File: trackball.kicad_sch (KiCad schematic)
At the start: 174 parts, among them J1 ZX-PM2.0-2-4PY, SW1 HX TC-5608-Y, SW2 HX TC-5608-Y, SW3 HX TC-5608-Y, SW4 HX TC-5608-Y, SW5 HX TC-5608-Y, SW6 HX TC-5608-Y, SW7 HX TC-5608-Y, SW8 HX TC-5608-Y, U1 SY8089A1AAC, U10 WS2812B, U11 WS2812B, U12 WS2812B, U13 WS2812B, U14 WS2812B, U15 WS2812B, U16 WS2812B, U17 WS2812B, U18 WS2812B, U19 WS2812B, U2 USB-TYPE-C-017, U20 WS2812B, U3 PMW3610, U4 PMW3610, U5 WS2812B, U6 WS2812B, U7 WS2812B, U8 WS2812B, U9 WS2812B, X1 XL7EL89CKI-111YLC-32M

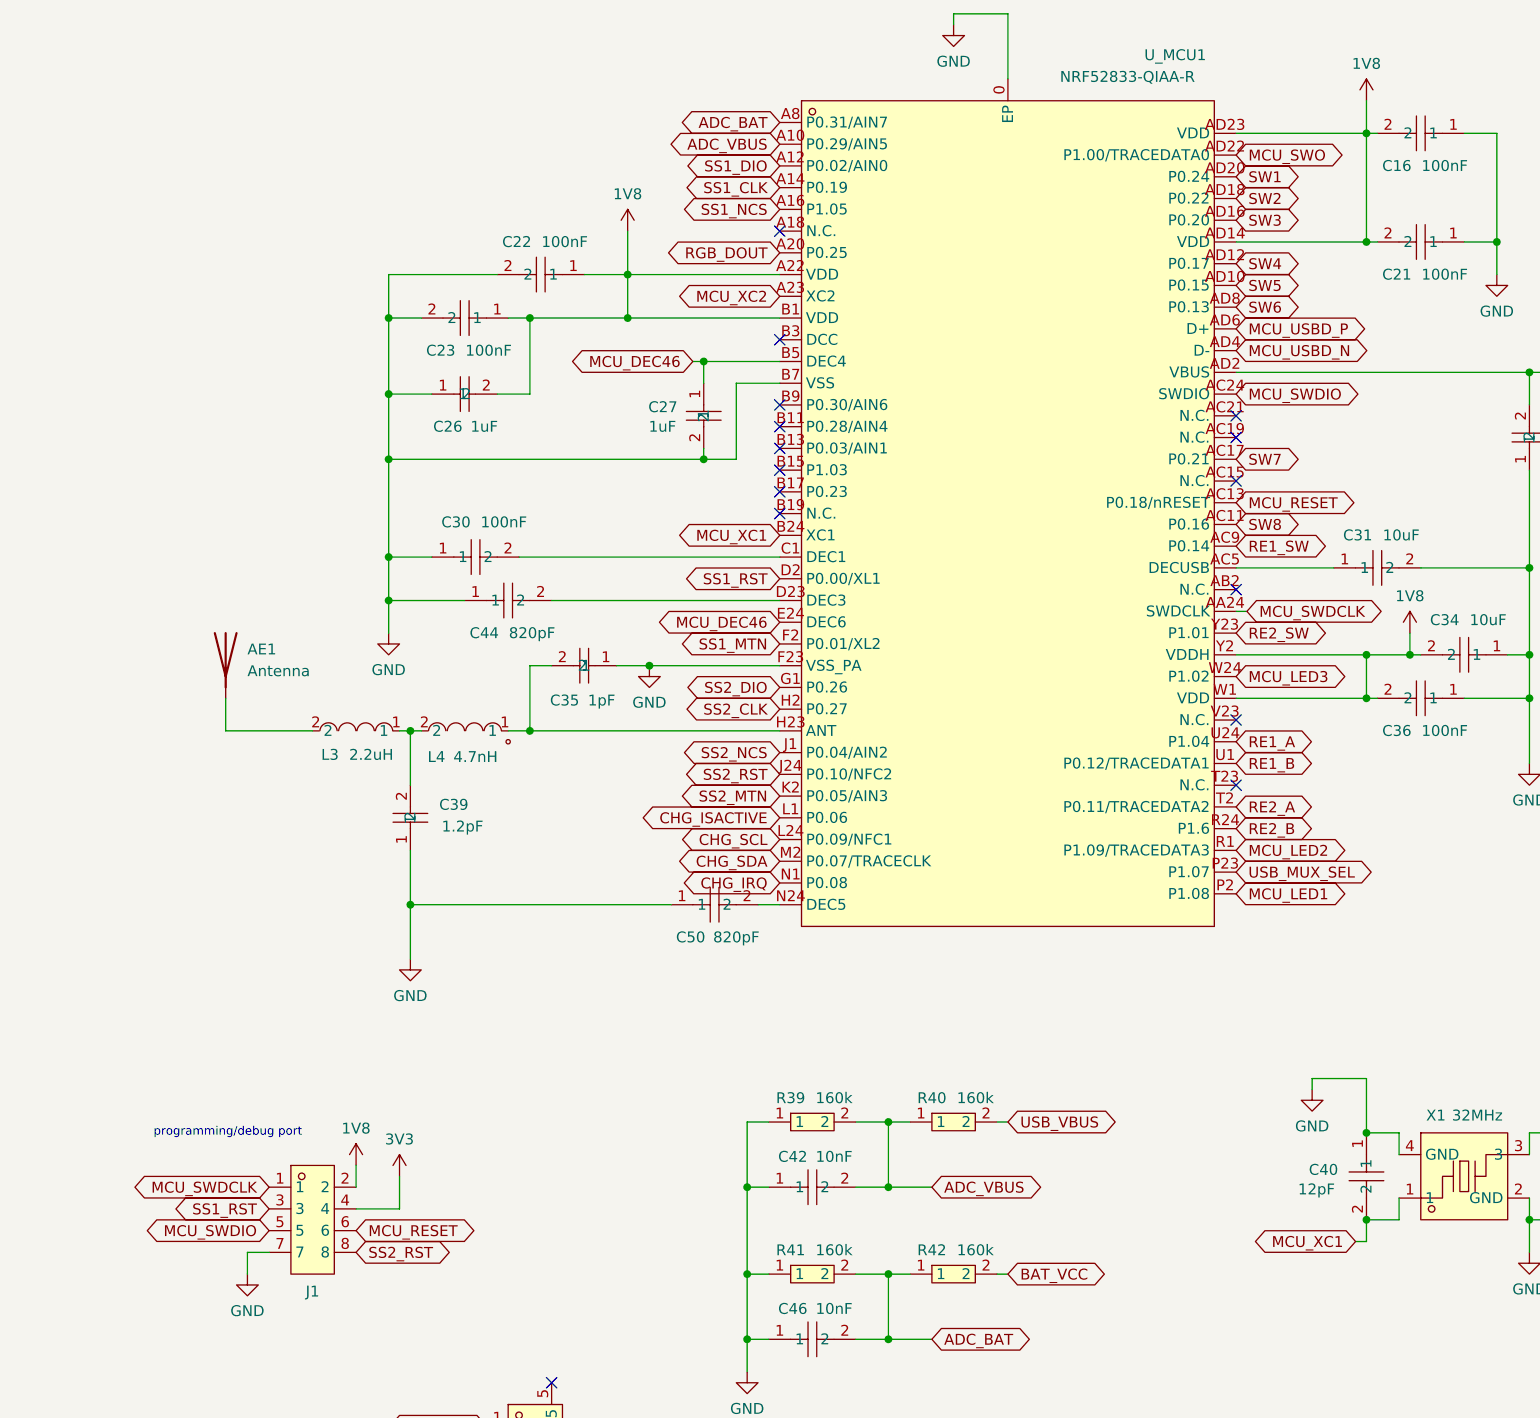
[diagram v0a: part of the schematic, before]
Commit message: chore: checkpoint
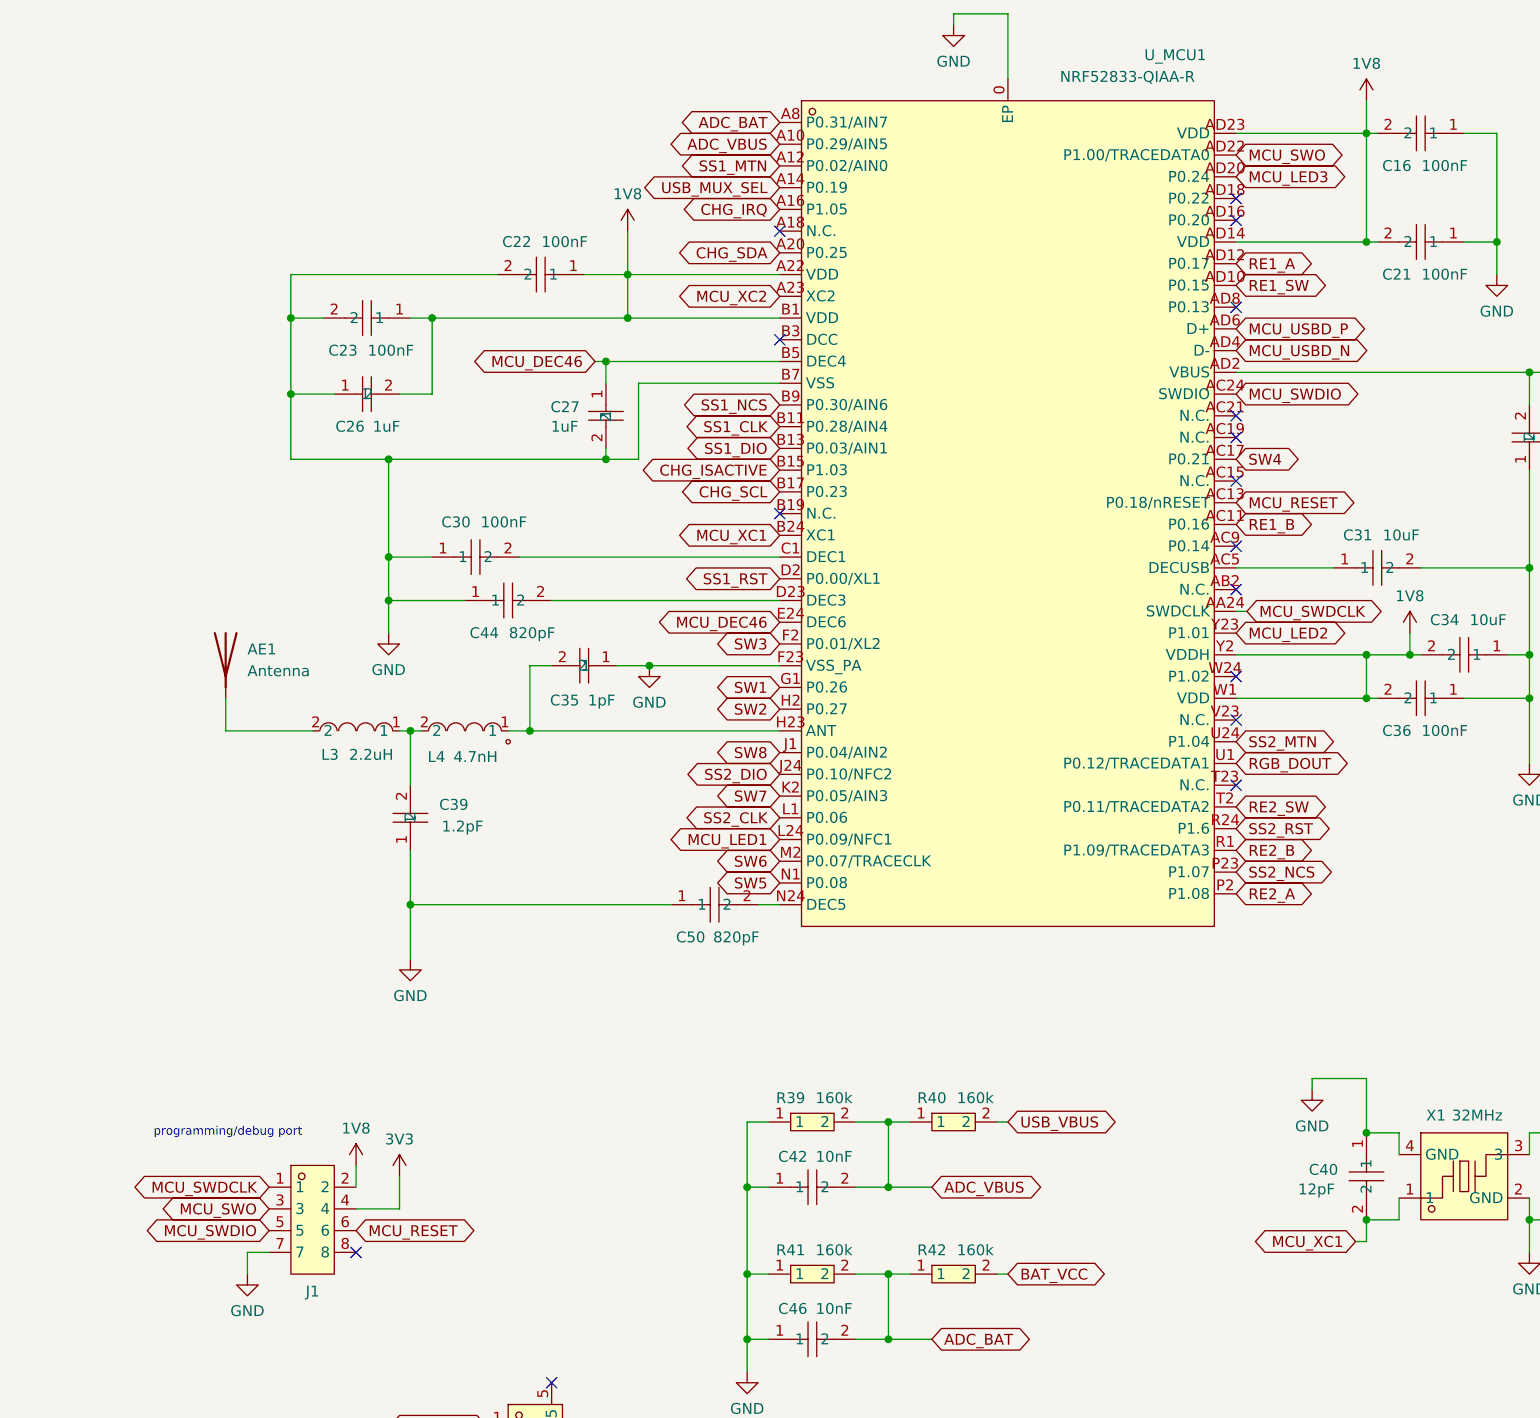
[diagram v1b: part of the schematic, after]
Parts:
- AE1: footprint antenna:Texas_SWRA117D_2.4GHz_Right -> antenna:Texas_SWRA117D_2.4GHz_Left
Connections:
- net CHG_IRQ: now also U_MCU1.A16 (P1.05); no longer U_MCU1.N1 (P0.08)
- net CHG_ISACTIVE: now also U_MCU1.B15 (P1.03); no longer U_MCU1.L1 (P0.06)
- net CHG_SCL: now also U_MCU1.B17 (P0.23); no longer U_MCU1.L24 (P0.09/NFC1)
- net CHG_SDA: now also U_MCU1.A20 (P0.25); no longer U_MCU1.M2 (P0.07/TRACECLK)
- net MCU_LED1: now also U_MCU1.L24 (P0.09/NFC1); no longer U_MCU1.P2 (P1.08)
- net MCU_LED2: now also U_MCU1.Y23 (P1.01); no longer U_MCU1.R1 (P1.09/TRACEDATA3)
- net MCU_LED3: now also U_MCU1.AD20 (P0.24); no longer U_MCU1.W24 (P1.02)
- net MCU_SWO: now also J1.3
- net RE1_A: now also U_MCU1.AD12 (P0.17); no longer U_MCU1.U24 (P1.04)
- net RE1_B: now also U_MCU1.AC11 (P0.16); no longer U_MCU1.U1 (P0.12/TRACEDATA1)
- net RE1_SW: now also U_MCU1.AD10 (P0.15); no longer U_MCU1.AC9 (P0.14)
- net RE2_A: now also U_MCU1.P2 (P1.08); no longer U_MCU1.T2 (P0.11/TRACEDATA2)
- net RE2_B: now also U_MCU1.R1 (P1.09/TRACEDATA3); no longer U_MCU1.R24 (P1.6)
- net RE2_SW: now also U_MCU1.T2 (P0.11/TRACEDATA2); no longer U_MCU1.Y23 (P1.01)
- net RGB_DOUT: now also U_MCU1.U1 (P0.12/TRACEDATA1); no longer U_MCU1.A20 (P0.25)
- net SS1_CLK: now also U_MCU1.B11 (P0.28/AIN4); no longer U_MCU1.A14 (P0.19)
- net SS1_DIO: now also U_MCU1.B13 (P0.03/AIN1); no longer U_MCU1.A12 (P0.02/AIN0)
- net SS1_MTN: now also U_MCU1.A12 (P0.02/AIN0); no longer U_MCU1.F2 (P0.01/XL2)
- net SS1_NCS: now also U_MCU1.B9 (P0.30/AIN6); no longer U_MCU1.A16 (P1.05)
- net SS1_RST: no longer J1.3
- net SS2_CLK: now also U_MCU1.L1 (P0.06); no longer U_MCU1.H2 (P0.27)
- net SS2_DIO: now also U_MCU1.J24 (P0.10/NFC2); no longer U_MCU1.G1 (P0.26)
- net SS2_MTN: now also U_MCU1.U24 (P1.04); no longer U_MCU1.K2 (P0.05/AIN3)
- net SS2_NCS: now also U_MCU1.P23 (P1.07); no longer U_MCU1.J1 (P0.04/AIN2)
- net SS2_RST: now also U_MCU1.R24 (P1.6); no longer J1.8, U_MCU1.J24 (P0.10/NFC2)
- net SW1: now also U_MCU1.G1 (P0.26); no longer U_MCU1.AD20 (P0.24)
- net SW2: now also U_MCU1.H2 (P0.27); no longer U_MCU1.AD18 (P0.22)
- net SW3: now also U_MCU1.F2 (P0.01/XL2); no longer U_MCU1.AD16 (P0.20)
- net SW4: now also U_MCU1.AC17 (P0.21); no longer U_MCU1.AD12 (P0.17)
- net SW5: now also U_MCU1.N1 (P0.08); no longer U_MCU1.AD10 (P0.15)
- net SW6: now also U_MCU1.M2 (P0.07/TRACECLK); no longer U_MCU1.AD8 (P0.13)
- net SW7: now also U_MCU1.K2 (P0.05/AIN3); no longer U_MCU1.AC17 (P0.21)
- net SW8: now also U_MCU1.J1 (P0.04/AIN2); no longer U_MCU1.AC11 (P0.16)
- net USB_MUX_SEL: now also U_MCU1.A14 (P0.19); no longer U_MCU1.P23 (P1.07)
- no-connect marks 52 -> 53
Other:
- moved on the sheet: C23, C26, C27
